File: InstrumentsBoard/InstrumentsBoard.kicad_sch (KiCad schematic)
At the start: 27 parts, among them J1 RJ45_LED_Shielded, Q1 BSS138, Q3 BSS138BK, U1 Teensy4.1_DEV-16771, U2 OKI

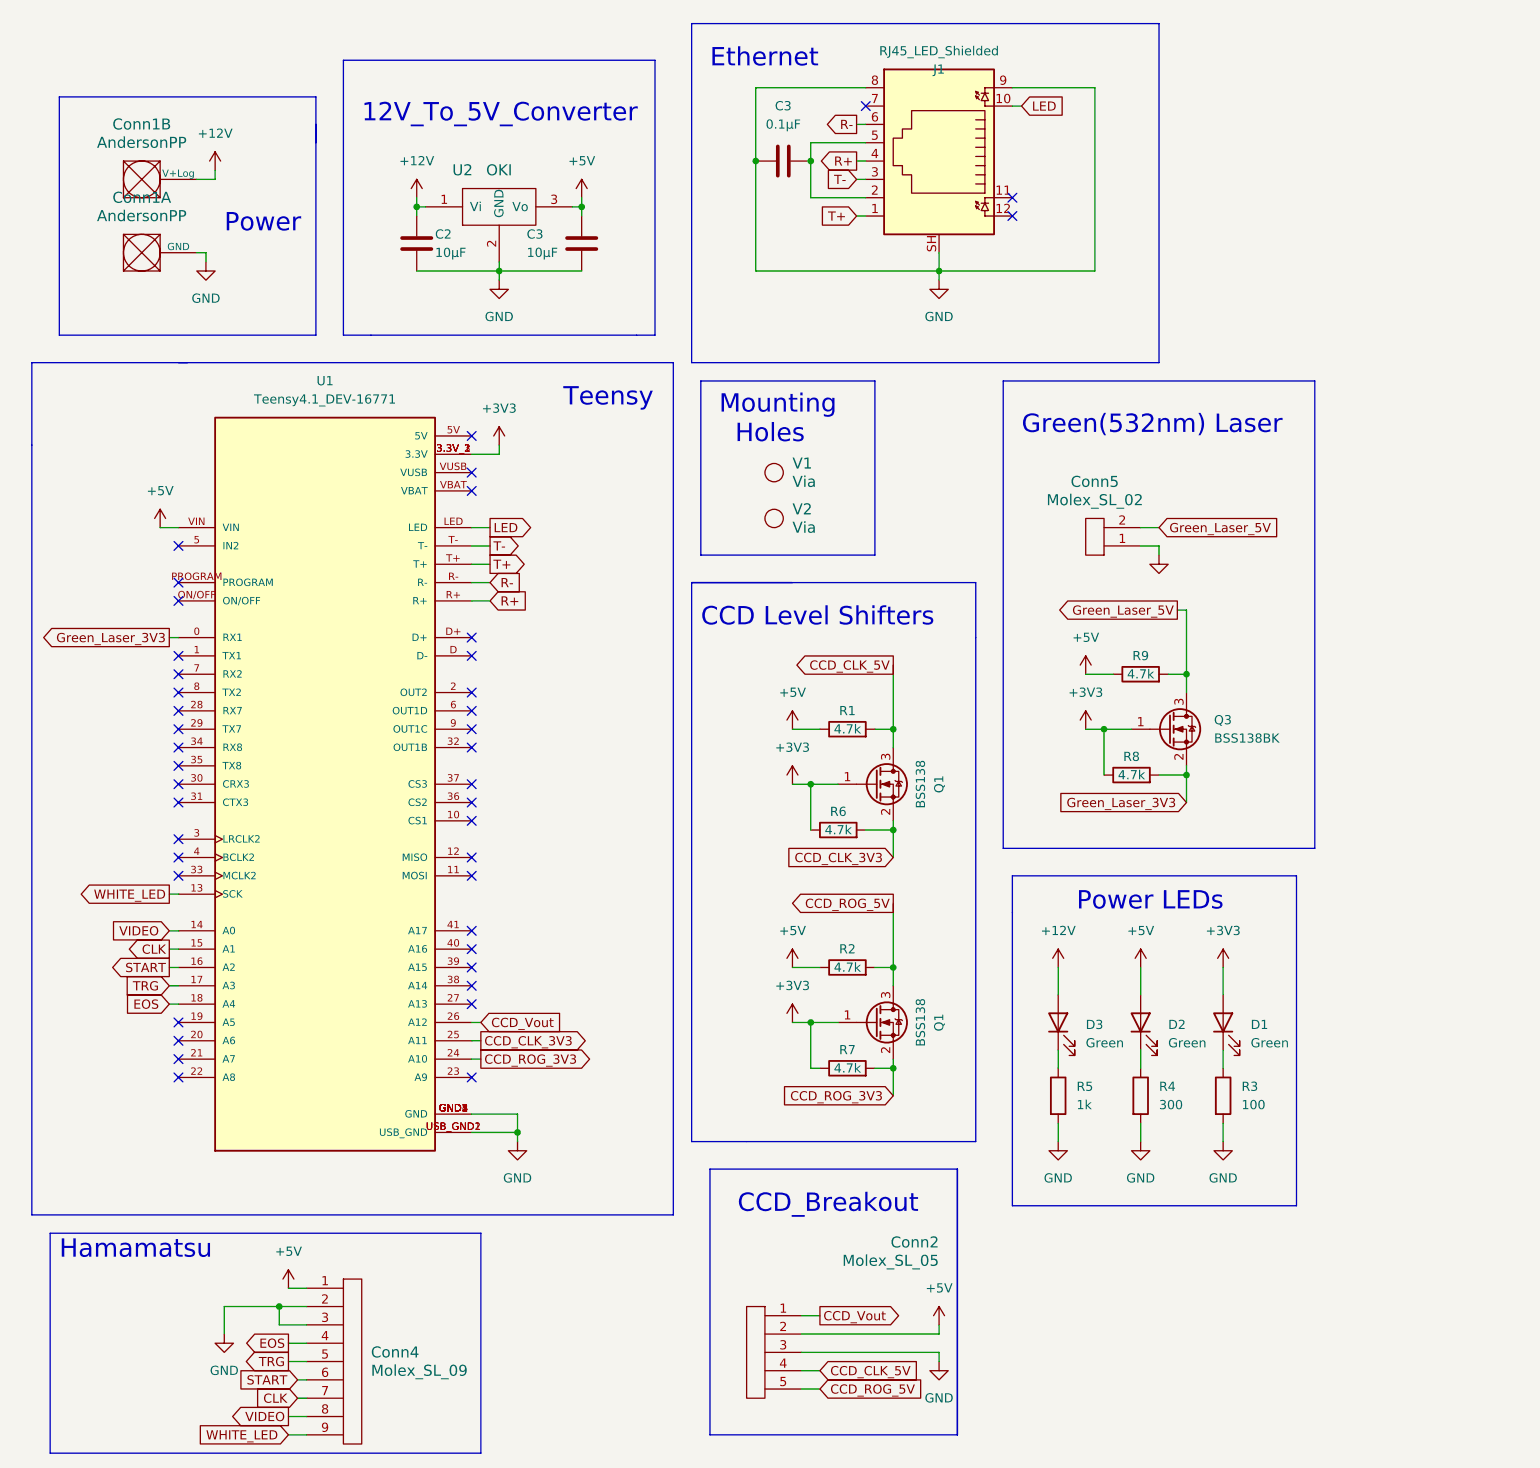
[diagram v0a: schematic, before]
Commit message: board review changes
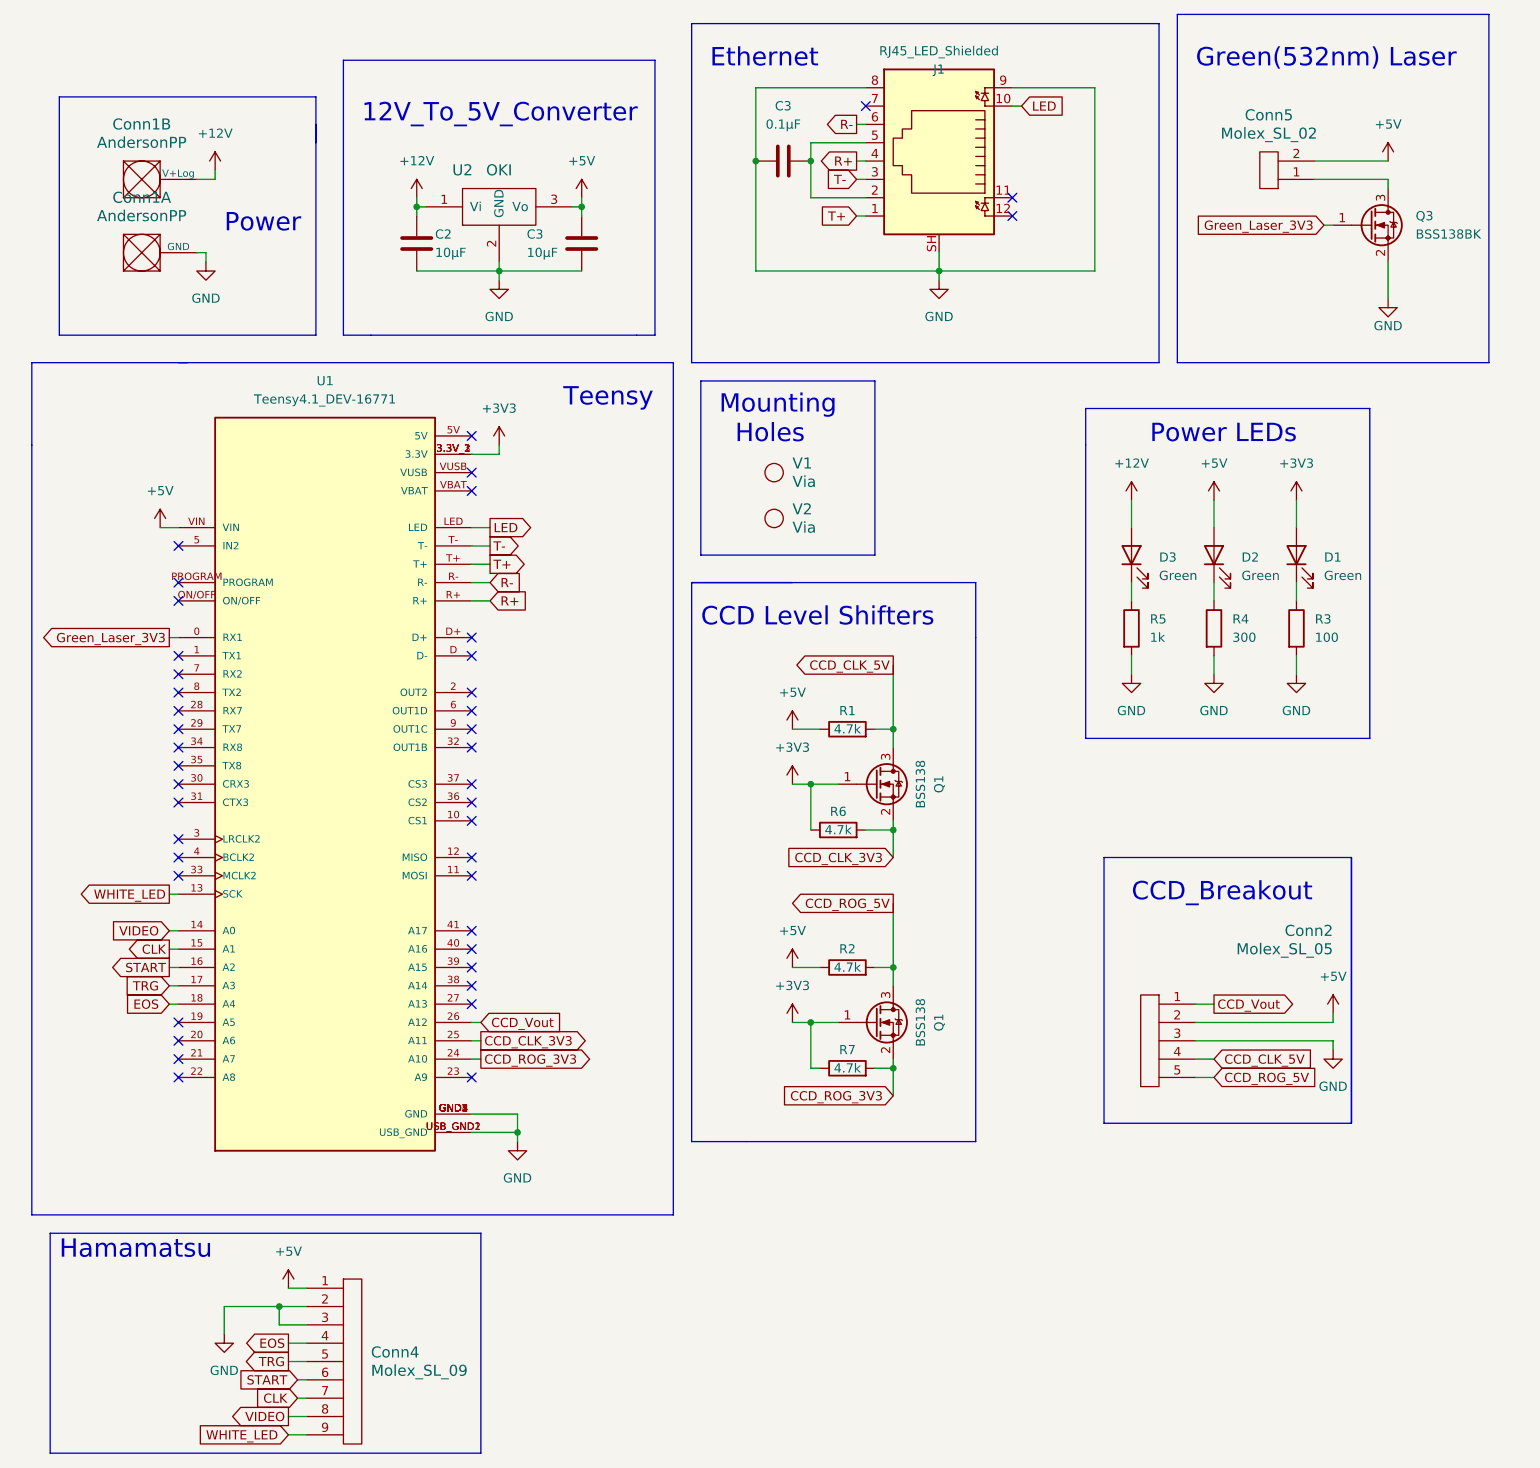
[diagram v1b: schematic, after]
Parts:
- removed R8, R9: 4.7k, Resistor_SMD:R_0603_1608Metric_Pad0.98x0.95mm_HandSolder, symbol Device:R
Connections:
- net +3V3: no longer Q3.1 (G)
- net +5V: now also Conn5.2
- net GND: now also Q3.2 (S); no longer Conn5.1
- net Green_Laser_3V3: now also Q3.1 (G); no longer Q3.2 (S)
- net Green_Laser_5V: no longer names the net of Q3.3 (D)
- net Green_Laser_5V: now also Conn5.1; no longer Conn5.2
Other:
- moved on the sheet: Conn2, Conn5, D1, D2, D3, Q3, R3, R4, R5

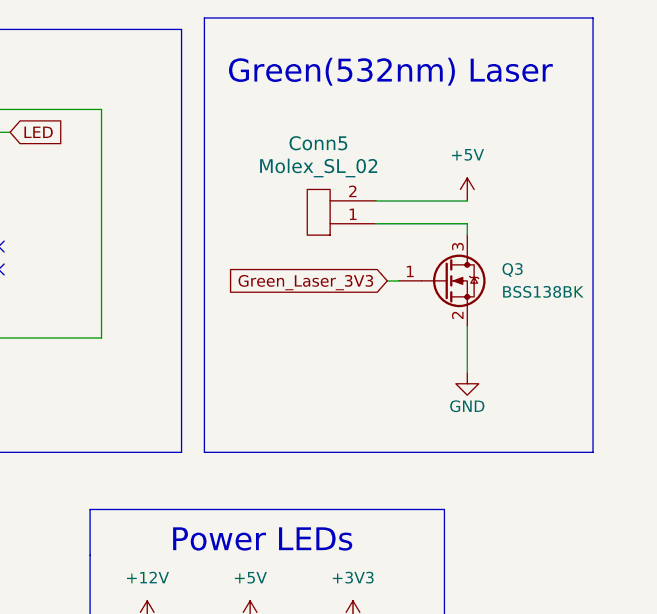
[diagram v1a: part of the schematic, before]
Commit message: fix low side toggle circuit
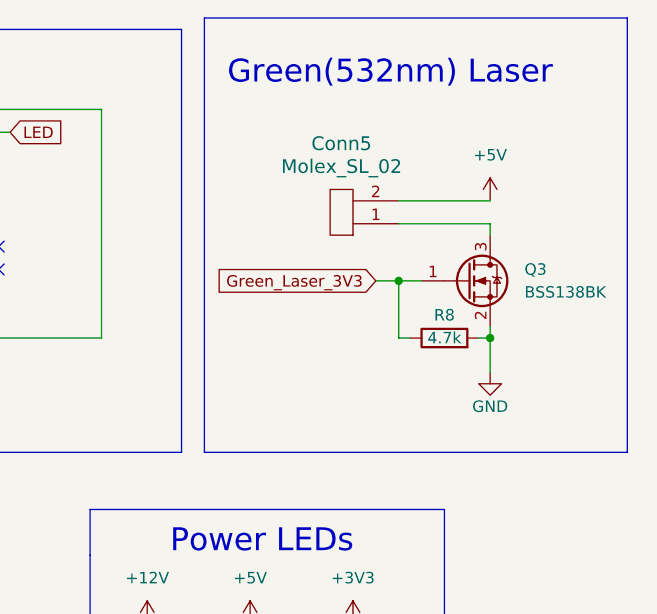
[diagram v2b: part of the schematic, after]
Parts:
- added R8: 4.7k, Resistor_SMD:R_0603_1608Metric_Pad0.98x0.95mm_HandSolder, symbol Device:R
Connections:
- net GND: now also R8.2
- net Green_Laser_3V3: now also R8.1
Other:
- moved on the sheet: Conn5, Q3
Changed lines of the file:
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@@
   (junction (at 91.44 41.91) (diameter 0) (color 0 0 0 0)
+  )
+  (junction (at 195.58 44.45) (diameter 0) (color 0 0 0 0)
+  )
+  (junction (at 205.74 50.8) (diameter 0) (color 0 0 0 0)
   )
   (junction (at 115.57 35.56) (diameter 0) (color 0 0 0 0)
@@
     (stroke (width 0) (type default))
   )
+  (wire (pts (xy 196.85 50.8) (xy 195.58 50.8))
+    (stroke (width 0) (type default))
+  )
   (wire (pts (xy 140.97 48.26) (xy 140.97 50.8))
     (stroke (width 0) (type default))
@@
     (stroke (width 0) (type default))
   )
-  (wire (pts (xy 203.2 38.1) (xy 203.2 39.37))
+  (wire (pts (xy 205.74 38.1) (xy 205.74 39.37))
     (stroke (width 0) (type default))
   )
@@
     (stroke (width 0) (type default))
   )
-  (polyline (pts (xy 173.99 15.24) (xy 217.17 15.24))
+  (polyline (pts (xy 173.99 15.24) (xy 220.98 15.24))
     (stroke (width 0) (type default))
   )
@@
     (stroke (width 0) (type default))
   )
-  (wire (pts (xy 194.31 44.45) (xy 195.58 44.45))
-    (stroke (width 0) (type default))
-  )
   (wire (pts (xy 167.64 93.98) (xy 167.64 96.52))
     (stroke (width 0) (type default))
@@
     (stroke (width 0) (type default))
   )
-  (wire (pts (xy 193.04 35.56) (xy 203.2 35.56))
+  (wire (pts (xy 195.58 35.56) (xy 205.74 35.56))
     (stroke (width 0) (type default))
   )
@@
     (stroke (width 0) (type default))
   )
+  (wire (pts (xy 204.47 50.8) (xy 205.74 50.8))
+    (stroke (width 0) (type default))
+  )
   (wire (pts (xy 68.58 50.8) (xy 80.01 50.8))
     (stroke (width 0) (type default))
@@
     (stroke (width 0) (type default))
   )
-  (wire (pts (xy 193.04 38.1) (xy 203.2 38.1))
+  (wire (pts (xy 195.58 38.1) (xy 205.74 38.1))
     (stroke (width 0) (type default))
   )
@@
     (stroke (width 0) (type default))
   )
+  (wire (pts (xy 205.74 50.8) (xy 205.74 54.61))
+    (stroke (width 0) (type default))
+  )
   (wire (pts (xy 176.53 154.94) (xy 195.58 154.94))
     (stroke (width 0) (type default))
@@
     (stroke (width 0) (type default))
   )
-  (wire (pts (xy 203.2 49.53) (xy 203.2 54.61))
+  (wire (pts (xy 205.74 49.53) (xy 205.74 50.8))
     (stroke (width 0) (type default))
   )
@@
     (stroke (width 0) (type default))
   )
+  (wire (pts (xy 195.58 44.45) (xy 198.12 44.45))
+    (stroke (width 0) (type default))
+  )
+  (wire (pts (xy 193.04 44.45) (xy 195.58 44.45))
+    (stroke (width 0) (type default))
+  )
   (wire (pts (xy 134.62 147.32) (xy 134.62 149.86))
     (stroke (width 0) (type default))
@@
     (stroke (width 0) (type default))
   )
-  (polyline (pts (xy 217.17 63.5) (xy 173.99 63.5))
+  (polyline (pts (xy 220.98 63.5) (xy 173.99 63.5))
     (stroke (width 0) (type default))
   )
@@
     (stroke (width 0) (type default))
   )
-  (polyline (pts (xy 217.17 15.24) (xy 217.17 63.5))
+  (polyline (pts (xy 220.98 15.24) (xy 220.98 63.5))
     (stroke (width 0) (type default))
   )
@@
   )
   (polyline (pts (xy 198.12 132.08) (xy 163.83 132.08))
+    (stroke (width 0) (type default))
+  )
+  (wire (pts (xy 195.58 50.8) (xy 195.58 44.45))
     (stroke (width 0) (type default))
   )
@@
     )
   )
-  (global_label "Green_Laser_3V3" (shape input) (at 194.31 44.45 180) (fields_autoplaced)
-    (effects (font (size 1.27 1.27)) (justify right))
-    (property "Intersheetrefs" "${INTERSHEET_REFS}" (at 175.4196 44.45 0)
+  (global_label "Green_Laser_3V3" (shape input) (at 193.04 44.45 180) (fields_autoplaced)
+    (effects (font (size 1.27 1.27)) (justify right))
+    (property "Intersheetrefs" "${INTERSHEET_REFS}" (at 174.1496 44.45 0)
       (effects (font (size 1.27 1.27)) (justify right) hide)
     )
@@
     )
   )
-  (symbol (lib_id "MRDT_Connectors:Molex_SL_02") (at 187.96 34.29 180) (unit 1)
-    (in_bom yes) (on_board yes) (dnp no) (fields_autoplaced)
-    (property "Reference" "Conn5" (at 186.69 29.21 0)
+  (symbol (lib_id "MRDT_Connectors:Molex_SL_02") (at 190.5 34.29 180) (unit 1)
+    (in_bom yes) (on_board yes) (dnp no) (fields_autoplaced)
+    (property "Reference" "Conn5" (at 189.23 29.21 0)
       (effects (font (size 1.524 1.524)))
     )
-    (property "Value" "Molex_SL_02" (at 186.69 31.75 0)
+    (property "Value" "Molex_SL_02" (at 189.23 31.75 0)
       (effects (font (size 1.524 1.524)))
     )
-    (property "Footprint" "MRDT_Connectors:MOLEX_SL_02_Vertical" (at 187.96 31.75 0)
+    (property "Footprint" "MRDT_Connectors:MOLEX_SL_02_Vertical" (at 190.5 31.75 0)
       (effects (font (size 1.524 1.524)) hide)
     )
-    (property "Datasheet" "" (at 187.96 31.75 0)
+    (property "Datasheet" "" (at 190.5 31.75 0)
       (effects (font (size 1.524 1.524)) hide)
     )
@@
     )
   )
-  (symbol (lib_id "Transistor_FET:BSS138") (at 200.66 44.45 0) (unit 1)
-    (in_bom yes) (on_board yes) (dnp no) (fields_autoplaced)
-    (property "Reference" "Q3" (at 207.01 43.18 0)
+  (symbol (lib_id "Transistor_FET:BSS138") (at 203.2 44.45 0) (unit 1)
+    (in_bom yes) (on_board yes) (dnp no) (fields_autoplaced)
+    (property "Reference" "Q3" (at 209.55 43.18 0)
       (effects (font (size 1.27 1.27)) (justify left))
     )
-    (property "Value" "BSS138BK" (at 207.01 45.72 0)
+    (property "Value" "BSS138BK" (at 209.55 45.72 0)
       (effects (font (size 1.27 1.27)) (justify left))
     )
-    (property "Footprint" "Package_TO_SOT_SMD:SOT-23" (at 205.74 46.355 0)
+    (property "Footprint" "Package_TO_SOT_SMD:SOT-23" (at 208.28 46.355 0)
       (effects (font (size 1.27 1.27) italic) (justify left) hide)
     )
-    (property "Datasheet" "https://www.onsemi.com/pub/Collateral/BSS138-D.PDF" (at 200.66 44.45 0)
+    (property "Datasheet" "https://www.onsemi.com/pub/Collateral/BSS138-D.PDF" (at 203.2 44.45 0)
       (effects (font (size 1.27 1.27)) (justify left) hide)
     )
@@
     )
   )
-  (symbol (lib_id "power:GND") (at 203.2 54.61 0) (unit 1)
+  (symbol (lib_id "power:GND") (at 205.74 54.61 0) (unit 1)
     (in_bom yes) (on_board yes) (dnp no)
-    (property "Reference" "#PWR09" (at 203.2 60.96 0)
-      (effects (font (size 1.27 1.27)) hide)
-    )
-    (property "Value" "GND" (at 203.2 58.42 0)
-      (effects (font (size 1.27 1.27)))
-    )
-    (property "Footprint" "" (at 203.2 54.61 0)
-      (effects (font (size 1.27 1.27)) hide)
-    )
-    (property "Datasheet" "" (at 203.2 54.61 0)
+    (property "Reference" "#PWR09" (at 205.74 60.96 0)
+      (effects (font (size 1.27 1.27)) hide)
+    )
+    (property "Value" "GND" (at 205.74 58.42 0)
+      (effects (font (size 1.27 1.27)))
+    )
+    (property "Footprint" "" (at 205.74 54.61 0)
+      (effects (font (size 1.27 1.27)) hide)
+    )
+    (property "Datasheet" "" (at 205.74 54.61 0)
       (effects (font (size 1.27 1.27)) hide)
     )
@@
     )
   )
-  (symbol (lib_id "power:+5V") (at 203.2 35.56 0) (unit 1)
-    (in_bom yes) (on_board yes) (dnp no) (fields_autoplaced)
-    (property "Reference" "#PWR016" (at 203.2 39.37 0)
-      (effects (font (size 1.27 1.27)) hide)
-    )
-    (property "Value" "+5V" (at 203.2 30.48 0)
-      (effects (font (size 1.27 1.27)))
-    )
-    (property "Footprint" "" (at 203.2 35.56 0)
-      (effects (font (size 1.27 1.27)) hide)
-    )
-    (property "Datasheet" "" (at 203.2 35.56 0)
+  (symbol (lib_id "power:+5V") (at 205.74 35.56 0) (unit 1)
+    (in_bom yes) (on_board yes) (dnp no) (fields_autoplaced)
+    (property "Reference" "#PWR016" (at 205.74 39.37 0)
+      (effects (font (size 1.27 1.27)) hide)
+    )
+    (property "Value" "+5V" (at 205.74 30.48 0)
+      (effects (font (size 1.27 1.27)))
+    )
+    (property "Footprint" "" (at 205.74 35.56 0)
+      (effects (font (size 1.27 1.27)) hide)
+    )
+    (property "Datasheet" "" (at 205.74 35.56 0)
       (effects (font (size 1.27 1.27)) hide)
     )
@@
         )
       )
+    )
+  )
+  (symbol (lib_id "Device:R") (at 200.66 50.8 90) (unit 1)
+    (in_bom yes) (on_board yes) (dnp no)
+    (property "Reference" "R8" (at 200.66 48.26 90)
+      (effects (font (size 1.27 1.27)))
+    )
+    (property "Value" "4.7k" (at 200.66 50.8 90)
+      (effects (font (size 1.27 1.27)))
+    )
+    (property "Footprint" "Resistor_SMD:R_0603_1608Metric_Pad0.98x0.95mm_HandSolder" (at 200.66 52.578 90)
+      (effects (font (size 1.27 1.27)) hide)
+    )
+    (property "Datasheet" "~" (at 200.66 50.8 0)
+      (effects (font (size 1.27 1.27)) hide)
+    )
+    (pin "1")
+    (pin "2")
+    (instances
+      (project "InstrumentsBoard"
+        (path "/dd57774e-6364-4f58-a24d-9970470de2f9"
+          (reference "R8") (unit 1)
+        )
+      )
